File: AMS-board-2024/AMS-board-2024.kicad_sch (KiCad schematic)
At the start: 54 parts, among them J1 XH_6pin_Side, J10 XH_6pin_Side, J11 XH_7pin_Side, J12 XH_6pin_Side, J13 XH_7pin_Side, J14 XH_6pin_Side, J15 XH_7pin_Side, J16 XH_6pin_Side, J17 XH_6pin_Side, J18 XH_6pin_Side, J19 19427-0040, J2 XH_7pin_Side, J20 19427-0040, J21 XH_6pin_Side, J22 XH_7pin_Side, J23 XH_6pin_Side, J24 XH_7pin_Side, J25 XH_6pin_Side, J26 XH_6pin_Side, J27 XH_2pin_Side, J28 XH_6pin_Side, J29 XH_5pin_Side, J3 XH_6pin_Side, J30 PinHeader_02x05_P1.00mm, J31 XH_2pin_Side, J32 5077CR-16-SMC2-BK-TR, J33 XH_5pin_Side, J4 XH_7pin_Side, J5 XH_6pin_Side, J6 XH_7pin_Side, J7 XH_6pin_Side, J8 XH_6pin_Side, J9 XH_6pin_Side

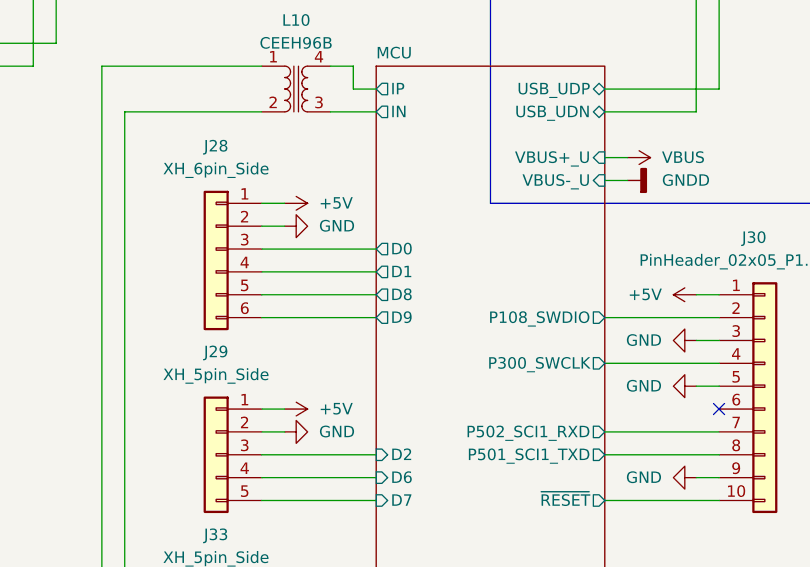
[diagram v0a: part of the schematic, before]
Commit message: 5V OUT のピンアサイン修正
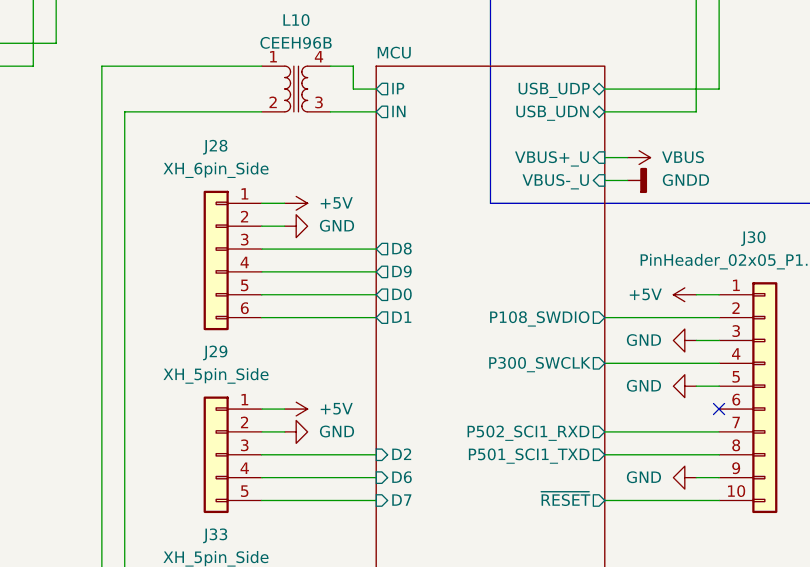
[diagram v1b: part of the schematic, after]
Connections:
- net MCU/D0: now also J28.5 (Pin_5); no longer J28.3 (Pin_3)
- net MCU/D1: now also J28.6 (Pin_6); no longer J28.4 (Pin_4)
- net MCU/D8: now also J28.3 (Pin_3); no longer J28.5 (Pin_5)
- net MCU/D9: now also J28.4 (Pin_4); no longer J28.6 (Pin_6)
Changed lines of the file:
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@@
       (effects (font (size 1.27 1.27)) (justify left))
     )
-    (pin "D9" output (at 317.5 154.94 180)
+    (pin "D9" output (at 317.5 149.86 180)
       (effects (font (size 1.27 1.27)) (justify left))
     )
-    (pin "D8" output (at 317.5 152.4 180)
+    (pin "D8" output (at 317.5 147.32 180)
       (effects (font (size 1.27 1.27)) (justify left))
     )
-    (pin "D1" output (at 317.5 149.86 180)
+    (pin "D1" output (at 317.5 154.94 180)
       (effects (font (size 1.27 1.27)) (justify left))
     )
-    (pin "D0" output (at 317.5 147.32 180)
+    (pin "D0" output (at 317.5 152.4 180)
       (effects (font (size 1.27 1.27)) (justify left))
     )

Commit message: 5V OUT ピンアサイン修正
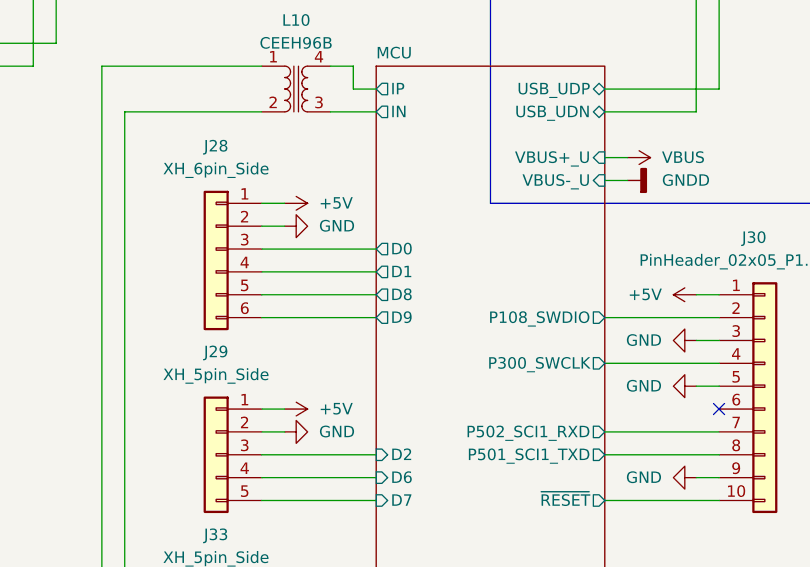
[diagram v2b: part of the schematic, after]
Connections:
- net MCU/D0: now also J28.3 (Pin_3); no longer J28.5 (Pin_5)
- net MCU/D1: now also J28.4 (Pin_4); no longer J28.6 (Pin_6)
- net MCU/D8: now also J28.5 (Pin_5); no longer J28.3 (Pin_3)
- net MCU/D9: now also J28.6 (Pin_6); no longer J28.4 (Pin_4)
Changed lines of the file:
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@@
       (effects (font (size 1.27 1.27)) (justify left))
     )
-    (pin "D9" output (at 317.5 149.86 180)
+    (pin "D9" output (at 317.5 154.94 180)
       (effects (font (size 1.27 1.27)) (justify left))
     )
-    (pin "D8" output (at 317.5 147.32 180)
+    (pin "D8" output (at 317.5 152.4 180)
       (effects (font (size 1.27 1.27)) (justify left))
     )
-    (pin "D1" output (at 317.5 154.94 180)
+    (pin "D1" output (at 317.5 149.86 180)
       (effects (font (size 1.27 1.27)) (justify left))
     )
-    (pin "D0" output (at 317.5 152.4 180)
+    (pin "D0" output (at 317.5 147.32 180)
       (effects (font (size 1.27 1.27)) (justify left))
     )

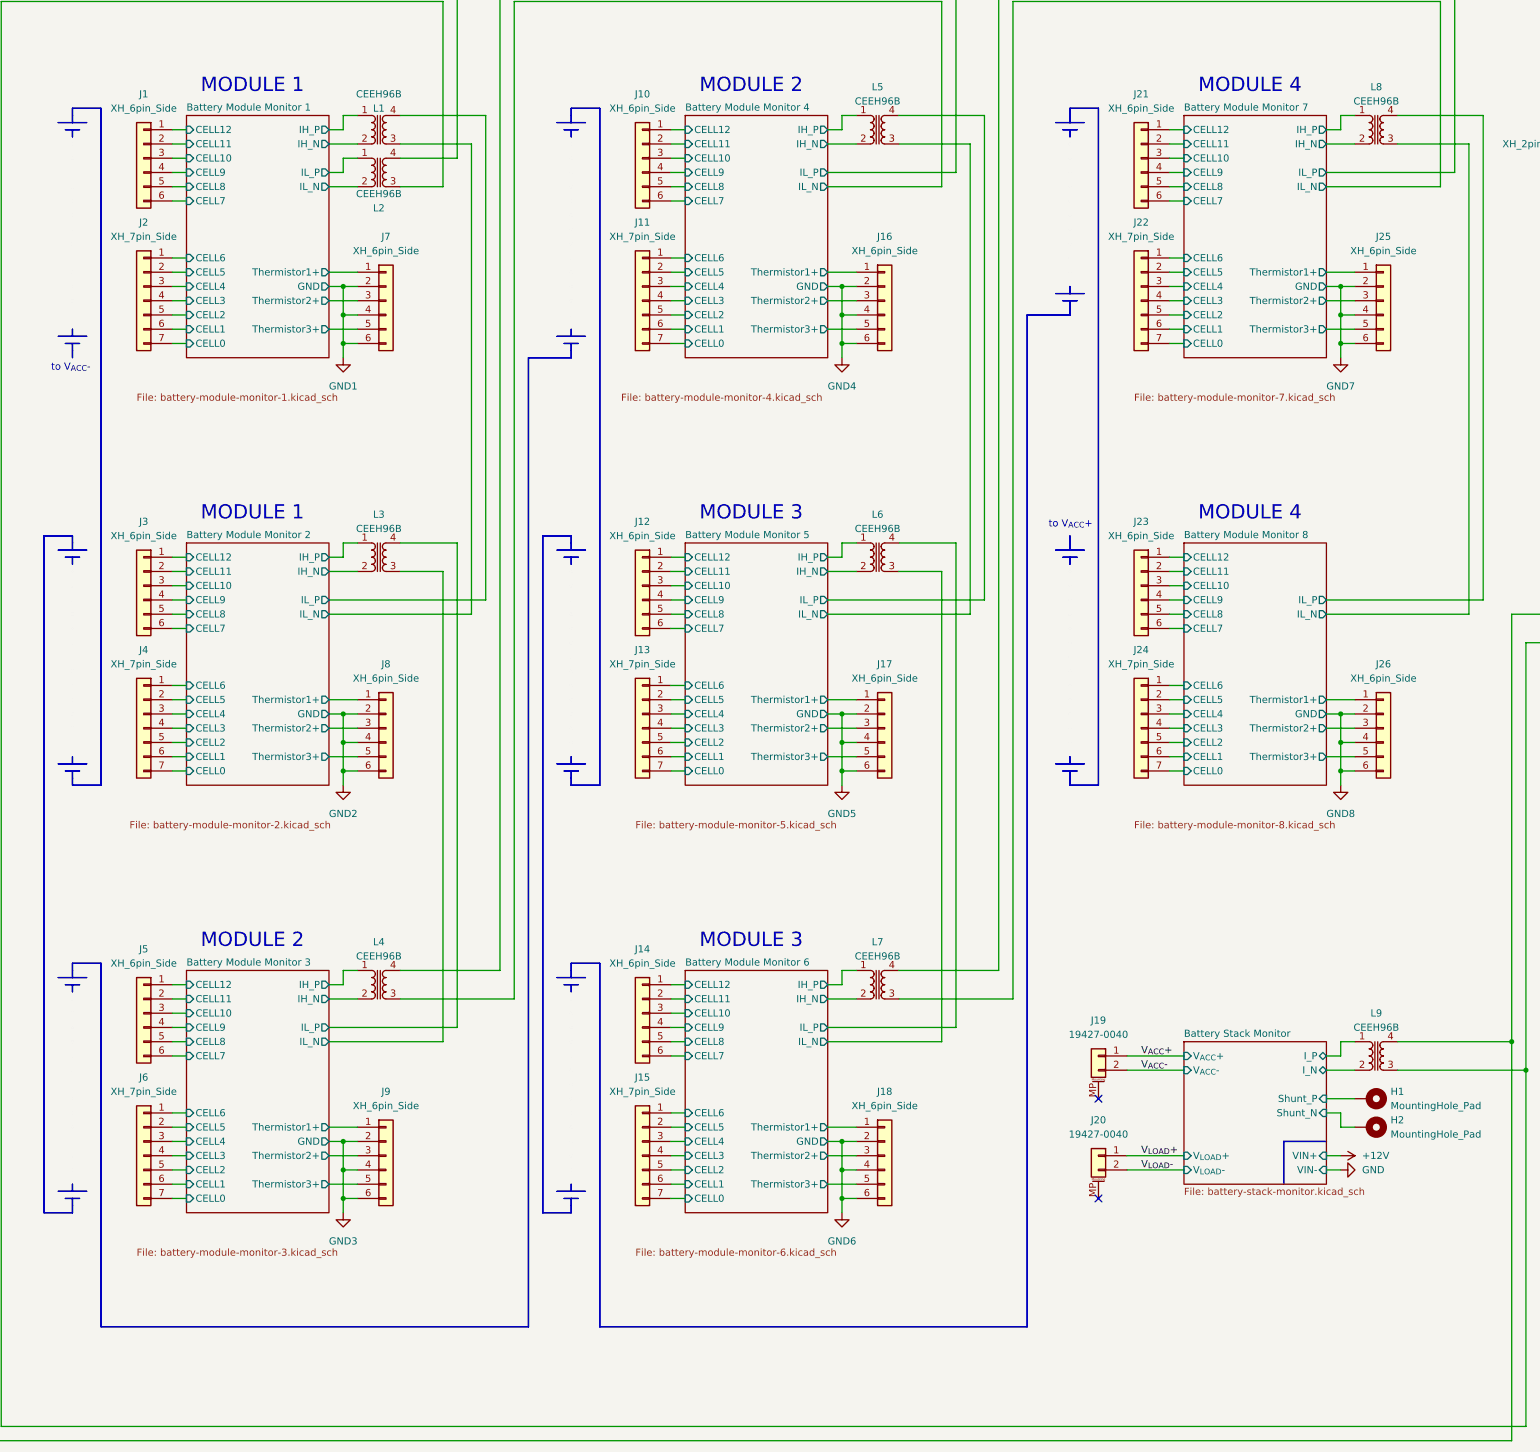
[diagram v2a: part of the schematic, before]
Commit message: セル監視用コネクタを表面実装XHに変更
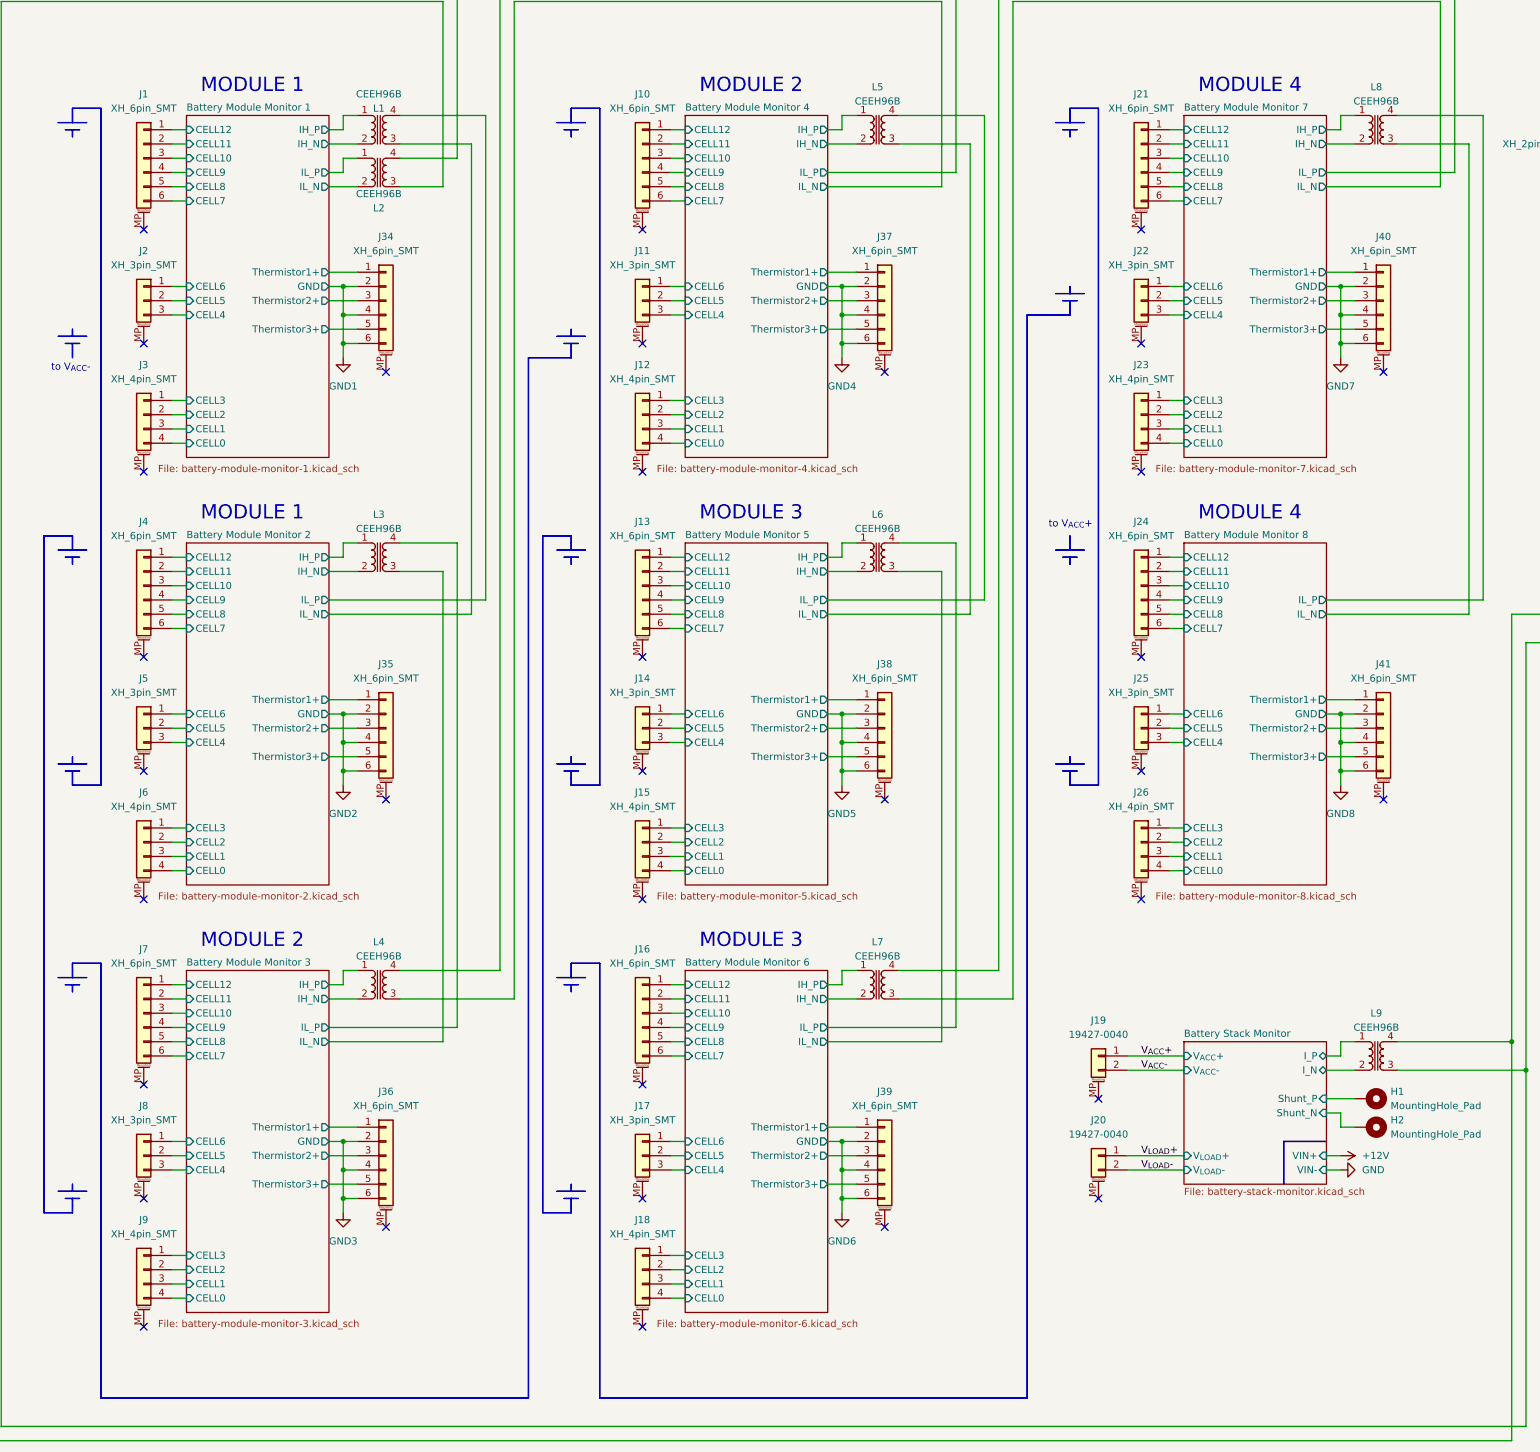
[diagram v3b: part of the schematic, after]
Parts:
- removed J1, J10, J12, J14, J16, J17, J18, J21, J23, J25, J26, J3, J5, J7, J8, J9: XH_6pin_Side, Connector_JST:JST_XH_S6B-XH-A_1x06_P2.50mm_Horizontal, symbol Connector_Generic:Conn_01x06
- removed J11, J13, J15, J2, J22, J24, J4, J6: XH_7pin_Side, Connector_JST:JST_XH_S7B-XH-A_1x07_P2.50mm_Horizontal, symbol Connector_Generic:Conn_01x07
- added J1, J10, J13, J16, J21, J24, J34, J35, J36, J37, J38, J39, J4, J40, J41, J7: XH_6pin_SMT, ProjectEV:Connector_S6B-XH-SM4-TB, symbol ProjectEV:Connector_XH_6pin_SMT
- added J11, J14, J17, J2, J22, J25, J5, J8: XH_3pin_SMT, ProjectEV:Connector_S3B-XH-SM4-TB, symbol ProjectEV:Connector_XH_3pin_SMT
- added J12, J15, J18, J23, J26, J3, J6, J9: XH_4pin_SMT, ProjectEV:Connector_S4B-XH-SM4-TB, symbol ProjectEV:Connector_XH_4pin_SMT
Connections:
- net Battery Module Monitor 1/CELL0: now also J3.4 (Pin_4)
- net Battery Module Monitor 1/CELL1: now also J3.3 (Pin_3)
- net Battery Module Monitor 1/CELL10: now also J1.3 (Pin_3)
- net Battery Module Monitor 1/CELL11: now also J1.2 (Pin_2)
- net Battery Module Monitor 1/CELL12: now also J1.1 (Pin_1)
- net Battery Module Monitor 1/CELL2: now also J3.2 (Pin_2)
- net Battery Module Monitor 1/CELL3: now also J3.1 (Pin_1)
- net Battery Module Monitor 1/CELL4: now also J2.3 (Pin_3)
- net Battery Module Monitor 1/CELL5: now also J2.2 (Pin_2)
- net Battery Module Monitor 1/CELL6: now also J2.1 (Pin_1)
- net Battery Module Monitor 1/CELL7: now also J1.6 (Pin_6)
- net Battery Module Monitor 1/CELL8: now also J1.5 (Pin_5)
- net Battery Module Monitor 1/CELL9: now also J1.4 (Pin_4)
- net Battery Module Monitor 1/Thermistor1+: now also J34.1 (Pin_1)
- net Battery Module Monitor 1/Thermistor2+: now also J34.3 (Pin_3)
- net Battery Module Monitor 1/Thermistor3+: now also J34.5 (Pin_5)
- net Battery Module Monitor 2/CELL0: now also J6.4 (Pin_4)
- net Battery Module Monitor 2/CELL1: now also J6.3 (Pin_3)
- net Battery Module Monitor 2/CELL10: now also J4.3 (Pin_3)
- net Battery Module Monitor 2/CELL11: now also J4.2 (Pin_2)
- net Battery Module Monitor 2/CELL12: now also J4.1 (Pin_1)
- net Battery Module Monitor 2/CELL2: now also J6.2 (Pin_2)
- net Battery Module Monitor 2/CELL3: now also J6.1 (Pin_1)
- net Battery Module Monitor 2/CELL4: now also J5.3 (Pin_3)
- net Battery Module Monitor 2/CELL5: now also J5.2 (Pin_2)
- net Battery Module Monitor 2/CELL6: now also J5.1 (Pin_1)
- net Battery Module Monitor 2/CELL7: now also J4.6 (Pin_6)
- net Battery Module Monitor 2/CELL8: now also J4.5 (Pin_5)
- net Battery Module Monitor 2/CELL9: now also J4.4 (Pin_4)
- net Battery Module Monitor 2/Thermistor1+: now also J35.1 (Pin_1)
- net Battery Module Monitor 2/Thermistor2+: now also J35.3 (Pin_3)
- net Battery Module Monitor 2/Thermistor3+: now also J35.5 (Pin_5)
- net Battery Module Monitor 3/CELL0: now also J9.4 (Pin_4)
- net Battery Module Monitor 3/CELL1: now also J9.3 (Pin_3)
- net Battery Module Monitor 3/CELL10: now also J7.3 (Pin_3)
- net Battery Module Monitor 3/CELL11: now also J7.2 (Pin_2)
- net Battery Module Monitor 3/CELL12: now also J7.1 (Pin_1)
- net Battery Module Monitor 3/CELL2: now also J9.2 (Pin_2)
- net Battery Module Monitor 3/CELL3: now also J9.1 (Pin_1)
- net Battery Module Monitor 3/CELL4: now also J8.3 (Pin_3)
- net Battery Module Monitor 3/CELL5: now also J8.2 (Pin_2)
- net Battery Module Monitor 3/CELL6: now also J8.1 (Pin_1)
- net Battery Module Monitor 3/CELL7: now also J7.6 (Pin_6)
- net Battery Module Monitor 3/CELL8: now also J7.5 (Pin_5)
- net Battery Module Monitor 3/CELL9: now also J7.4 (Pin_4)
- net Battery Module Monitor 3/Thermistor1+: now also J36.1 (Pin_1)
- net Battery Module Monitor 3/Thermistor2+: now also J36.3 (Pin_3)
- net Battery Module Monitor 3/Thermistor3+: now also J36.5 (Pin_5)
- net Battery Module Monitor 4/CELL0: now also J12.4 (Pin_4)
- net Battery Module Monitor 4/CELL1: now also J12.3 (Pin_3)
- net Battery Module Monitor 4/CELL10: now also J10.3 (Pin_3)
- net Battery Module Monitor 4/CELL11: now also J10.2 (Pin_2)
- net Battery Module Monitor 4/CELL12: now also J10.1 (Pin_1)
- net Battery Module Monitor 4/CELL2: now also J12.2 (Pin_2)
- net Battery Module Monitor 4/CELL3: now also J12.1 (Pin_1)
- net Battery Module Monitor 4/CELL4: now also J11.3 (Pin_3)
- net Battery Module Monitor 4/CELL5: now also J11.2 (Pin_2)
- net Battery Module Monitor 4/CELL6: now also J11.1 (Pin_1)
- net Battery Module Monitor 4/CELL7: now also J10.6 (Pin_6)
- net Battery Module Monitor 4/CELL8: now also J10.5 (Pin_5)
- net Battery Module Monitor 4/CELL9: now also J10.4 (Pin_4)
- net Battery Module Monitor 4/Thermistor1+: now also J37.1 (Pin_1)
- net Battery Module Monitor 4/Thermistor2+: now also J37.3 (Pin_3)
- net Battery Module Monitor 4/Thermistor3+: now also J37.5 (Pin_5)
- net Battery Module Monitor 5/CELL0: now also J15.4 (Pin_4)
- net Battery Module Monitor 5/CELL1: now also J15.3 (Pin_3)
- net Battery Module Monitor 5/CELL10: now also J13.3 (Pin_3)
- net Battery Module Monitor 5/CELL11: now also J13.2 (Pin_2)
- net Battery Module Monitor 5/CELL12: now also J13.1 (Pin_1)
- net Battery Module Monitor 5/CELL2: now also J15.2 (Pin_2)
- net Battery Module Monitor 5/CELL3: now also J15.1 (Pin_1)
- net Battery Module Monitor 5/CELL4: now also J14.3 (Pin_3)
- net Battery Module Monitor 5/CELL5: now also J14.2 (Pin_2)
- net Battery Module Monitor 5/CELL6: now also J14.1 (Pin_1)
- net Battery Module Monitor 5/CELL7: now also J13.6 (Pin_6)
- net Battery Module Monitor 5/CELL8: now also J13.5 (Pin_5)
- net Battery Module Monitor 5/CELL9: now also J13.4 (Pin_4)
- net Battery Module Monitor 5/Thermistor1+: now also J38.1 (Pin_1)
- net Battery Module Monitor 5/Thermistor2+: now also J38.3 (Pin_3)
- net Battery Module Monitor 5/Thermistor3+: now also J38.5 (Pin_5)
- net Battery Module Monitor 6/CELL0: now also J18.4 (Pin_4)
- net Battery Module Monitor 6/CELL1: now also J18.3 (Pin_3)
- net Battery Module Monitor 6/CELL10: now also J16.3 (Pin_3)
- net Battery Module Monitor 6/CELL11: now also J16.2 (Pin_2)
- net Battery Module Monitor 6/CELL12: now also J16.1 (Pin_1)
- net Battery Module Monitor 6/CELL2: now also J18.2 (Pin_2)
- net Battery Module Monitor 6/CELL3: now also J18.1 (Pin_1)
- net Battery Module Monitor 6/CELL4: now also J17.3 (Pin_3)
- net Battery Module Monitor 6/CELL5: now also J17.2 (Pin_2)
- net Battery Module Monitor 6/CELL6: now also J17.1 (Pin_1)
- net Battery Module Monitor 6/CELL7: now also J16.6 (Pin_6)
- net Battery Module Monitor 6/CELL8: now also J16.5 (Pin_5)
- net Battery Module Monitor 6/CELL9: now also J16.4 (Pin_4)
- net Battery Module Monitor 6/Thermistor1+: now also J39.1 (Pin_1)
- net Battery Module Monitor 6/Thermistor2+: now also J39.3 (Pin_3)
- net Battery Module Monitor 6/Thermistor3+: now also J39.5 (Pin_5)
- net Battery Module Monitor 7/CELL0: now also J23.4 (Pin_4)
- net Battery Module Monitor 7/CELL1: now also J23.3 (Pin_3)
- net Battery Module Monitor 7/CELL10: now also J21.3 (Pin_3)
- net Battery Module Monitor 7/CELL11: now also J21.2 (Pin_2)
- net Battery Module Monitor 7/CELL12: now also J21.1 (Pin_1)
- net Battery Module Monitor 7/CELL2: now also J23.2 (Pin_2)
- net Battery Module Monitor 7/CELL3: now also J23.1 (Pin_1)
- net Battery Module Monitor 7/CELL4: now also J22.3 (Pin_3)
- net Battery Module Monitor 7/CELL5: now also J22.2 (Pin_2)
- net Battery Module Monitor 7/CELL6: now also J22.1 (Pin_1)
- net Battery Module Monitor 7/CELL7: now also J21.6 (Pin_6)
- net Battery Module Monitor 7/CELL8: now also J21.5 (Pin_5)
- net Battery Module Monitor 7/CELL9: now also J21.4 (Pin_4)
- net Battery Module Monitor 7/Thermistor1+: now also J40.1 (Pin_1)
- net Battery Module Monitor 7/Thermistor2+: now also J40.3 (Pin_3)
- net Battery Module Monitor 7/Thermistor3+: now also J40.5 (Pin_5)
- net Battery Module Monitor 8/CELL0: now also J26.4 (Pin_4)
- net Battery Module Monitor 8/CELL1: now also J26.3 (Pin_3)
- net Battery Module Monitor 8/CELL10: now also J24.3 (Pin_3)
- net Battery Module Monitor 8/CELL11: now also J24.2 (Pin_2)
- net Battery Module Monitor 8/CELL12: now also J24.1 (Pin_1)
- net Battery Module Monitor 8/CELL2: now also J26.2 (Pin_2)
- net Battery Module Monitor 8/CELL3: now also J26.1 (Pin_1)
- net Battery Module Monitor 8/CELL4: now also J25.3 (Pin_3)
- net Battery Module Monitor 8/CELL5: now also J25.2 (Pin_2)
- net Battery Module Monitor 8/CELL6: now also J25.1 (Pin_1)
- net Battery Module Monitor 8/CELL7: now also J24.6 (Pin_6)
- net Battery Module Monitor 8/CELL8: now also J24.5 (Pin_5)
- net Battery Module Monitor 8/CELL9: now also J24.4 (Pin_4)
- net Battery Module Monitor 8/Thermistor1+: now also J41.1 (Pin_1)
- net Battery Module Monitor 8/Thermistor2+: now also J41.3 (Pin_3)
- net Battery Module Monitor 8/Thermistor3+: now also J41.5 (Pin_5)
- net GND1: now also J34.2 (Pin_2), J34.4 (Pin_4), J34.6 (Pin_6)
- net GND2: now also J35.2 (Pin_2), J35.4 (Pin_4), J35.6 (Pin_6)
- net GND3: now also J36.2 (Pin_2), J36.4 (Pin_4), J36.6 (Pin_6)
- net GND4: now also J37.2 (Pin_2), J37.4 (Pin_4), J37.6 (Pin_6)
- net GND5: now also J38.2 (Pin_2), J38.4 (Pin_4), J38.6 (Pin_6)
- net GND6: now also J39.2 (Pin_2), J39.4 (Pin_4), J39.6 (Pin_6)
- net GND7: now also J40.2 (Pin_2), J40.4 (Pin_4), J40.6 (Pin_6)
- net GND8: now also J41.2 (Pin_2), J41.4 (Pin_4), J41.6 (Pin_6)
- no-connect marks 10 -> 42
